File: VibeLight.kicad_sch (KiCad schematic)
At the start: 14 parts, among them SW1 SW_Push, SW2 SW_Push

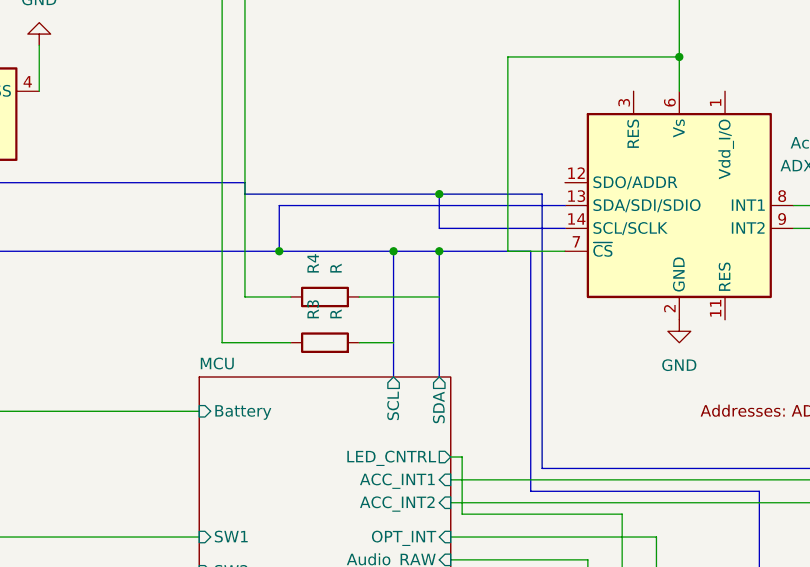
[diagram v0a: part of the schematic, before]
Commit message: completed rev1 of PCB layout
need to double check components and other elements, connections, and add values
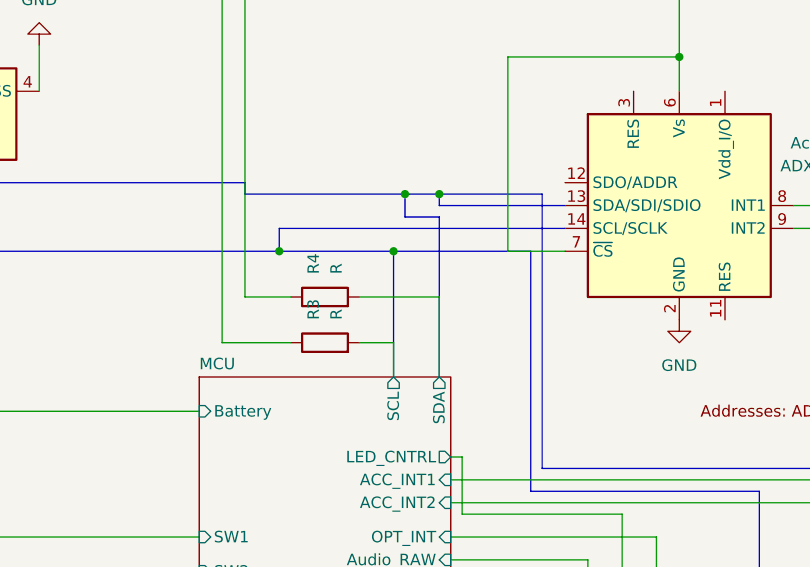
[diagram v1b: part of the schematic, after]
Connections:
- net MCU/SCL: now also R3.2
- net MCU/SDA: now also R4.2
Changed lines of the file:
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@@
 (kicad_sch (version 20230121) (generator eeschema)
   (paper "A4")
-  (junction (at 142.24 80.01) (diameter 0) (color 0 0 0 0)
-  )
   (junction (at 30.48 106.68) (diameter 0) (color 0 0 0 0)
   )
@@
   (junction (at 212.09 49.53) (diameter 0) (color 0 0 0 0)
   )
+  (junction (at 138.43 73.66) (diameter 0) (color 0 0 0 0)
+  )
   (junction (at 27.94 107.95) (diameter 0) (color 0 0 0 0)
   )
@@
     (stroke (width 0) (type default))
   )
-  (bus (pts (xy 142.24 80.01) (xy 152.4 80.01))
-    (stroke (width 0) (type default))
-  )
-  (bus (pts (xy 124.46 74.93) (xy 124.46 80.01))
+  (bus (pts (xy 124.46 77.47) (xy 124.46 80.01))
     (stroke (width 0) (type default))
   )
@@
     (stroke (width 0) (type default))
   )
-  (bus (pts (xy 137.16 80.01) (xy 142.24 80.01))
+  (bus (pts (xy 137.16 80.01) (xy 152.4 80.01))
     (stroke (width 0) (type default))
   )
@@
     (stroke (width 0) (type default))
   )
+  (wire (pts (xy 137.16 90.17) (xy 137.16 93.98))
+    (stroke (width 0) (type default))
+  )
   (bus (pts (xy 92.71 72.39) (xy 120.65 72.39))
     (stroke (width 0) (type default))
@@
     (stroke (width 0) (type default))
   )
+  (bus (pts (xy 142.24 93.98) (xy 142.24 76.2))
+    (stroke (width 0) (type default))
+  )
   (wire (pts (xy 27.94 106.68) (xy 30.48 106.68))
     (stroke (width 0) (type default))
@@
     (stroke (width 0) (type default))
   )
+  (wire (pts (xy 142.24 85.09) (xy 142.24 93.98))
+    (stroke (width 0) (type default))
+  )
   (wire (pts (xy 227.33 124.46) (xy 166.37 124.46))
     (stroke (width 0) (type default))
@@
     (stroke (width 0) (type default))
   )
-  (bus (pts (xy 120.65 73.66) (xy 142.24 73.66))
+  (bus (pts (xy 120.65 73.66) (xy 138.43 73.66))
     (stroke (width 0) (type default))
   )
@@
     (stroke (width 0) (type default))
   )
-  (bus (pts (xy 156.21 74.93) (xy 124.46 74.93))
+  (bus (pts (xy 156.21 77.47) (xy 124.46 77.47))
     (stroke (width 0) (type default))
   )
@@
     (stroke (width 0) (type default))
   )
-  (bus (pts (xy 142.24 77.47) (xy 156.21 77.47))
+  (bus (pts (xy 142.24 74.93) (xy 156.21 74.93))
     (stroke (width 0) (type default))
   )
@@
     (stroke (width 0) (type default))
   )
+  (bus (pts (xy 142.24 76.2) (xy 138.43 76.2))
+    (stroke (width 0) (type default))
+  )
   (wire (pts (xy 133.35 85.09) (xy 142.24 85.09))
     (stroke (width 0) (type default))
@@
     (stroke (width 0) (type default))
   )
+  (bus (pts (xy 138.43 73.66) (xy 142.24 73.66))
+    (stroke (width 0) (type default))
+  )
   (bus (pts (xy 87.63 80.01) (xy 124.46 80.01))
     (stroke (width 0) (type default))
@@
     (stroke (width 0) (type default))
   )
-  (bus (pts (xy 142.24 80.01) (xy 142.24 93.98))
+  (bus (pts (xy 138.43 73.66) (xy 138.43 76.2))
     (stroke (width 0) (type default))
   )
@@
     (stroke (width 0) (type default))
   )
-  (bus (pts (xy 142.24 77.47) (xy 142.24 73.66))
-    (stroke (width 0) (type default))
-  )
+  (bus (pts (xy 142.24 74.93) (xy 142.24 73.66))
+    (stroke (width 0) (type default))
+  )

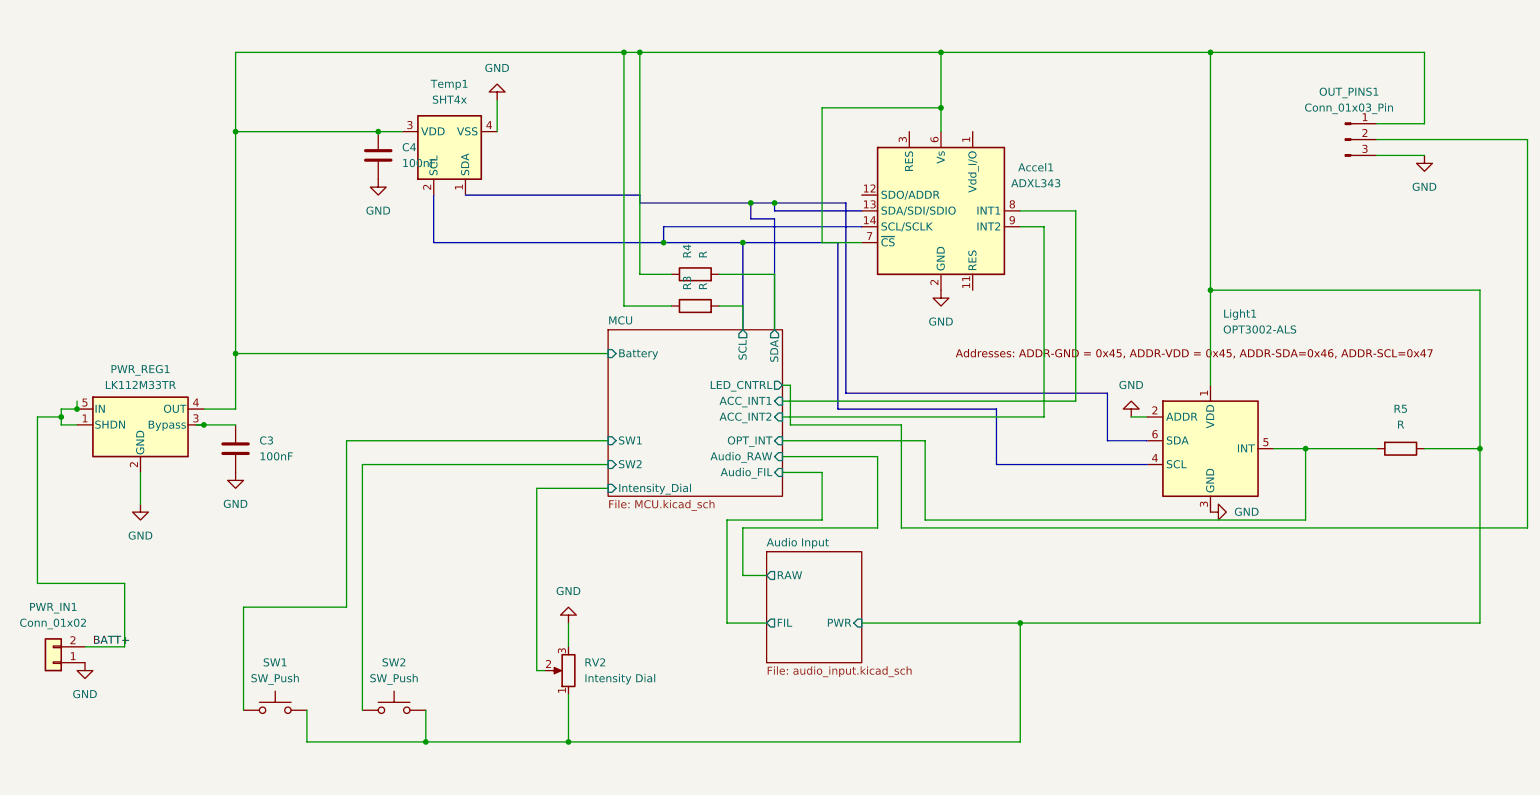
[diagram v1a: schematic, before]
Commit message: Changes from DR call
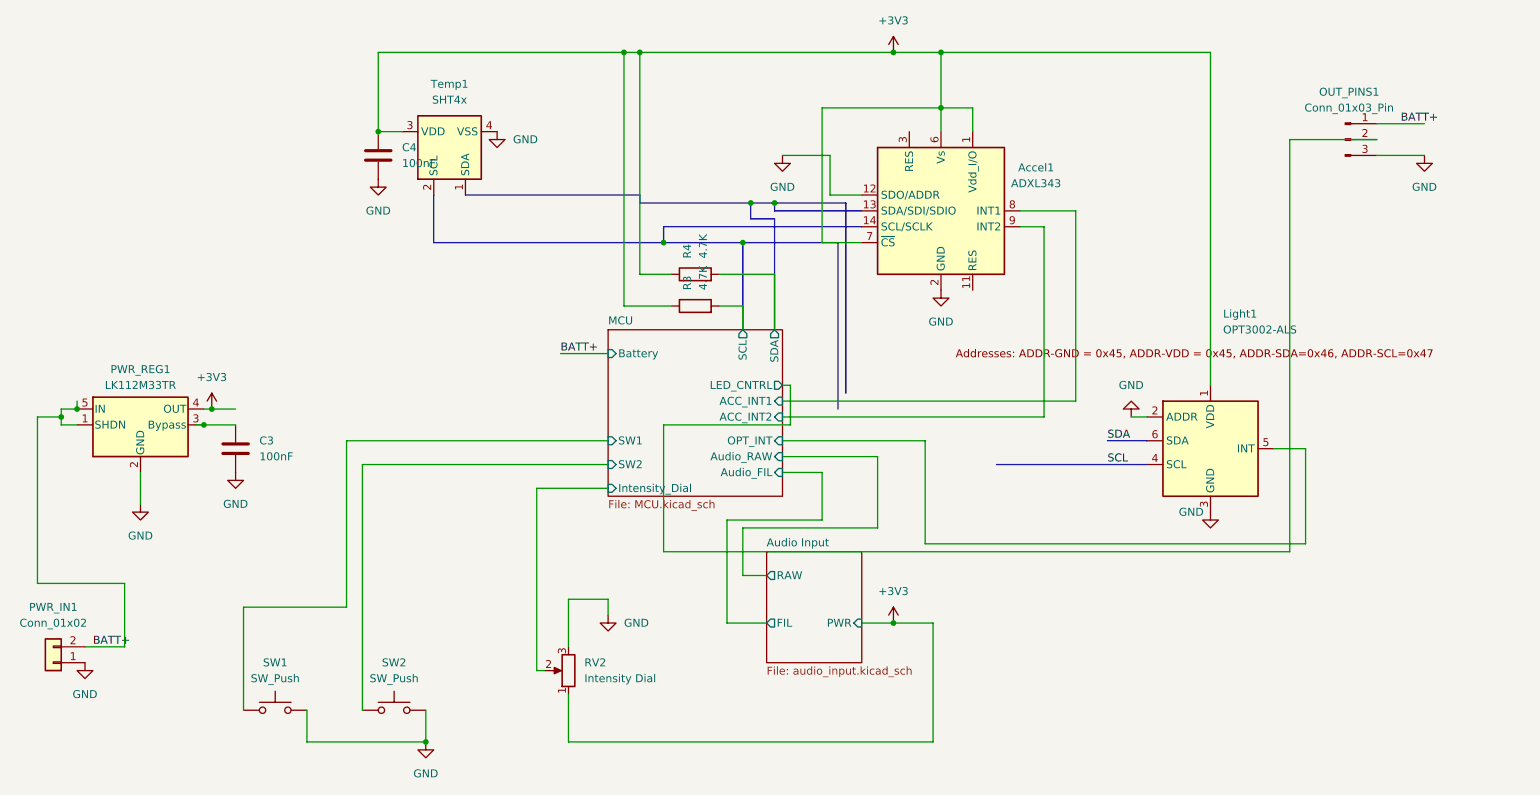
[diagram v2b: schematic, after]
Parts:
- removed R5: R, Resistor_SMD:R_0603_1608Metric_Pad0.98x0.95mm_HandSolder, symbol Device:R
- R3, R4: value R -> 4.7K
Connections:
- net BATT+: now also OUT_PINS1.1 (Pin_1)
- net GND: now also Accel1.12 (SDO/ADDR), SW1.2, SW2.2
- net +3V3: now reaches Accel1.1 (Vdd_I/O)
- net +3V3: now also Accel1.6 (Vs), Accel1.7 (~{CS}), C4.1, Light1.1 (VDD), PWR_REG1.4 (OUT), R3.1, R4.1, RV2.1, Temp1.3 (VDD)
- removed net Audio Input/PWR: Accel1.6 (Vs), Accel1.7 (~{CS}), C4.1, Light1.1 (VDD), OUT_PINS1.1 (Pin_1), PWR_REG1.4 (OUT), R3.1, R4.1, RV2.1, SW1.2, SW2.2, Temp1.3 (VDD)
